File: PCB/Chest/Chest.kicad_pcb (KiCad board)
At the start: 2 copper layers, 70 x 70 mm, 62 parts, among them J1 Reset, J10 L, J11 R, J12 TF_PUSH, J2 A, J3 B, J4 TC2030-USB-NL-DS, J5 USB-C-Socket-H, J6 1, J7 2, J8 3, J9 4, U1 MD8942, U2 ESP32-S3-MINI-1, U3 L, U4 R, U5 MAX98357A, U6 MAX98357A

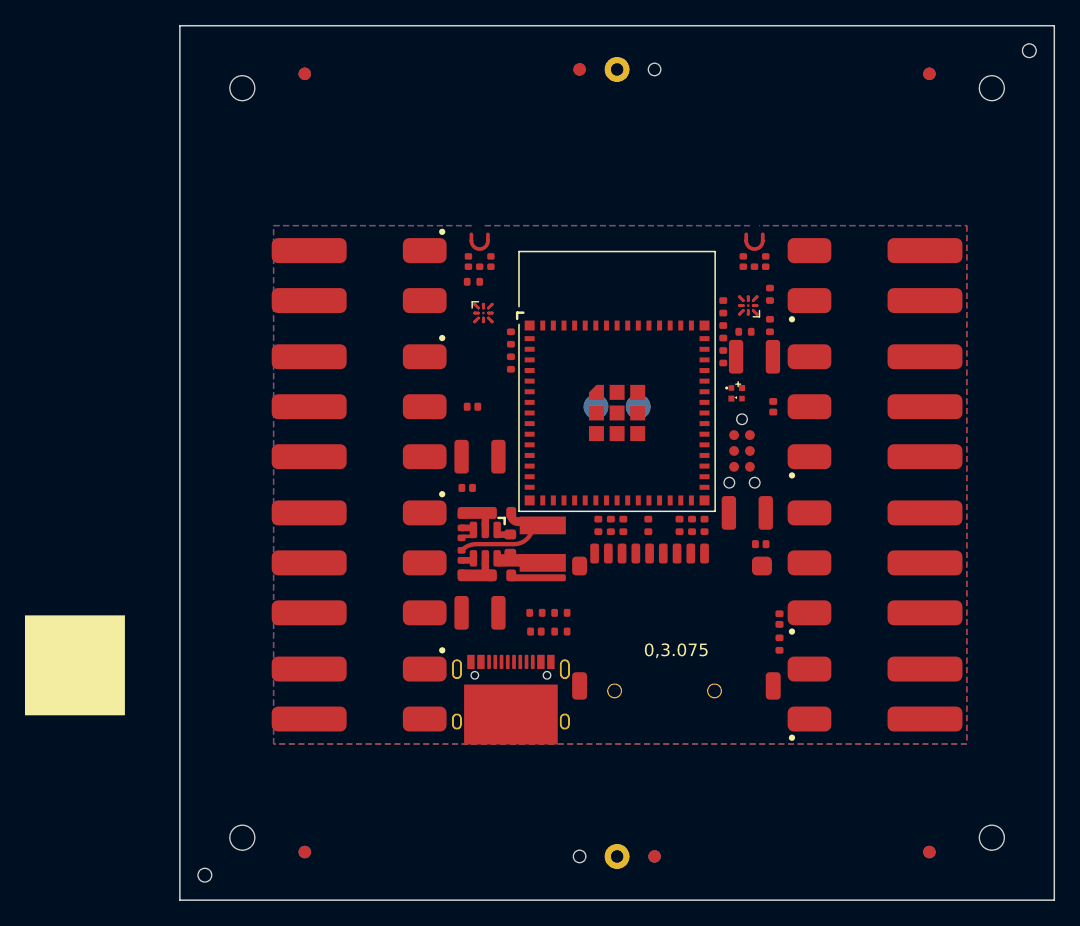
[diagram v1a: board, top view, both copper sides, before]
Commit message: Bigger caps
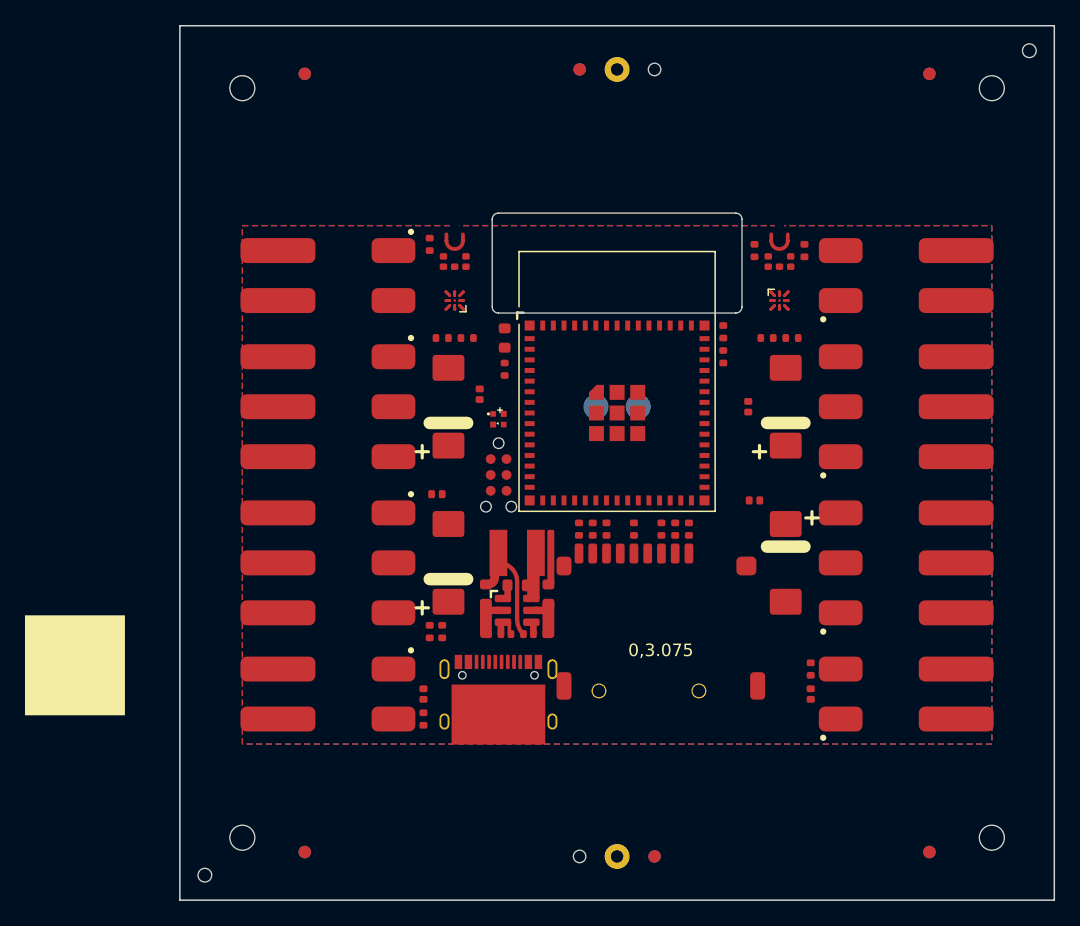
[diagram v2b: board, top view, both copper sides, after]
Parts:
- added C15: 100nF, RevK:C_0402, F.Cu at (91.0, 92.5)
- added C16: 22uF, RevK:C_0603, F.Cu at (91.0, 90.0)
- C5, C6, C7, C8: value 22uF 35V -> C_Polarized; footprint RevK:C_1210 -> RevK:CP_EIA-7343-31_Kemet-D
- moved C11 26.3 mm to (86.0, 90.0), turned to 180 degrees
- moved C14 20.5 mm to (112.0, 90.0), turned to 180 degrees
- moved J4 19.6 mm to (90.5, 101.0)
- moved D3 19.2 mm to (90.5, 96.5)
- moved R4 13.0 mm to (84.5, 120.5), turned to -90 degrees
- moved D1 10.3 mm to (84.5, 118.5), turned to 90 degrees
- moved R8 9.62 mm to (86.0, 113.5), turned to -90 degrees
- moved R2 9.38 mm to (90.2, 113.7), turned to 180 degrees
- moved R7 8.63 mm to (85.0, 113.5), turned to 90 degrees
- moved R1 8.46 mm to (92.0, 113.7), turned to 180 degrees
- moved R3 8.26 mm to (93.8, 113.7), turned to 180 degrees
- moved R16 7.91 mm to (115.0, 83.0)
- moved C2 6.62 mm to (89.5, 110.5), turned to -90 degrees
- moved D2 6.50 mm to (115.5, 118.5), turned to -90 degrees
- moved U1 5.88 mm to (92.0, 111.8), turned to 180 degrees
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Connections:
- C5 pad 1: GND -> DC
- C5 pad 2: DC -> GND
- C6 pad 1: GND -> DC
- C6 pad 2: DC -> GND
- C7 pad 1: GND -> DC
- C7 pad 2: DC -> GND
- C8 pad 1: GND -> DC
- C8 pad 2: DC -> GND
- U2 pad 10: unconnected-(U2-GPIO6-Pad10) -> LED1
- U2 pad 11: LED0 -> LED3
- U2 pad 12: LED1 -> unconnected-(U2-GPIO8-Pad12)
- U2 pad 13: LED2 -> unconnected-(U2-GPIO9-Pad13)
- U2 pad 14: LED3 -> unconnected-(U2-GPIO10-Pad14)
- U2 pad 15: LED4 -> unconnected-(U2-GPIO11-Pad15)
- U2 pad 16: SDDAT2 -> BTNA
- U2 pad 17: SDDAT3 -> BTNB
- U2 pad 18: SDCMD -> unconnected-(U2-GPIO14-Pad18)
- U2 pad 19: SDCLK -> unconnected-(U2-GPIO15-Pad19)
- U2 pad 20: SDDAT0 -> unconnected-(U2-GPIO16-Pad20)
- U2 pad 21: SDDAT1 -> unconnected-(U2-GPIO17-Pad21)
- U2 pad 22: SDCD -> unconnected-(U2-GPIO18-Pad22)
- U2 pad 27: unconnected-(U2-GPIO47-Pad27) -> SDCD
- U2 pad 28: BTNA -> SDDAT1
- U2 pad 29: BTNB -> SDDAT0
- U2 pad 31: unconnected-(U2-GPIO35-Pad31) -> SDCLK
- U2 pad 32: unconnected-(U2-GPIO36-Pad32) -> SDCMD
- U2 pad 33: unconnected-(U2-GPIO37-Pad33) -> SDDAT3
- U2 pad 34: unconnected-(U2-GPIO38-Pad34) -> SDDAT2
- U2 pad 36: MICWS -> unconnected-(U2-GPIO40-Pad36)
- U2 pad 37: MICSD -> LED4
- U2 pad 38: MICSCK -> LED2
- U2 pad 39: unconnected-(U2-GPIO43-Pad39) -> MICSD
- U2 pad 40: SPKPWR -> MICSCK
- U2 pad 44: unconnected-(U2-GPIO46-Pad44) -> MICWS
- U2 pad 8: LED2 -> SPKPWR
- U2 pad 9: unconnected-(U2-GPIO5-Pad9) -> LED0
